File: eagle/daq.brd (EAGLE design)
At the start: 76.2 x 65.4 mm, 109 parts

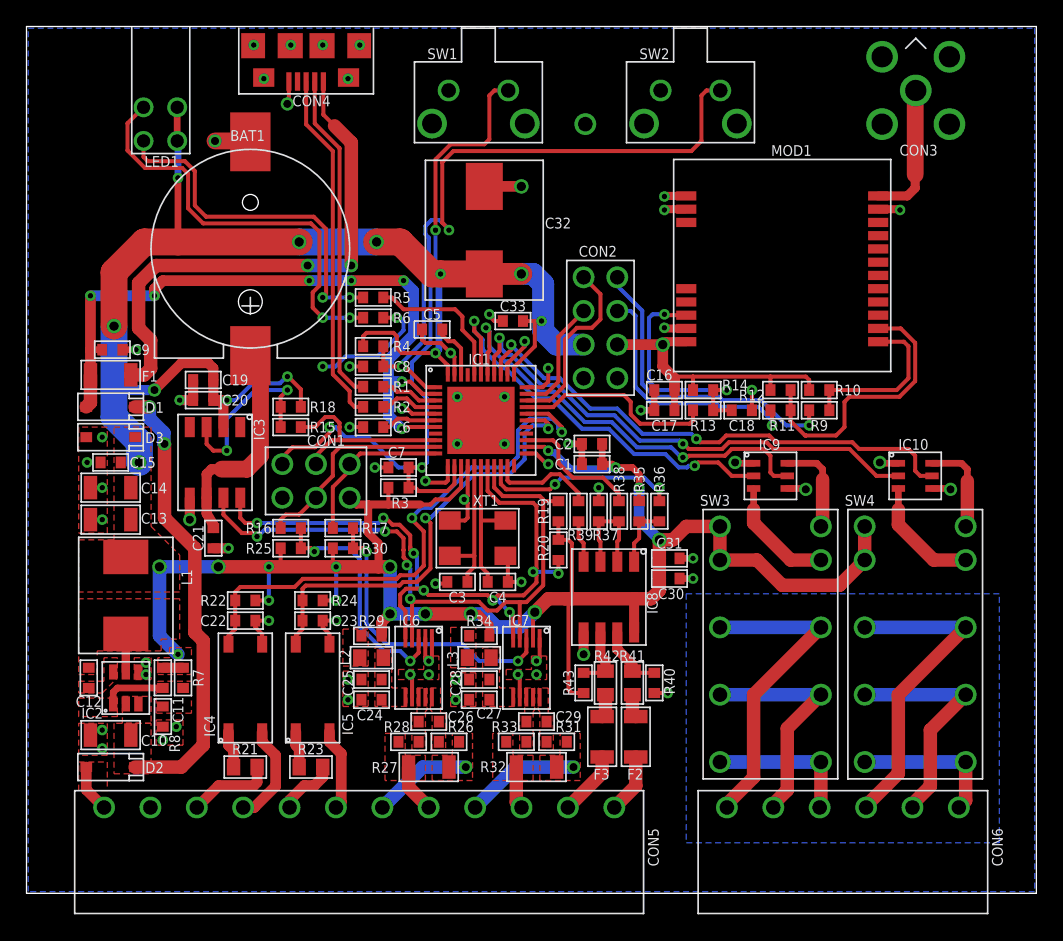
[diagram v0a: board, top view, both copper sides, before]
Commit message: do
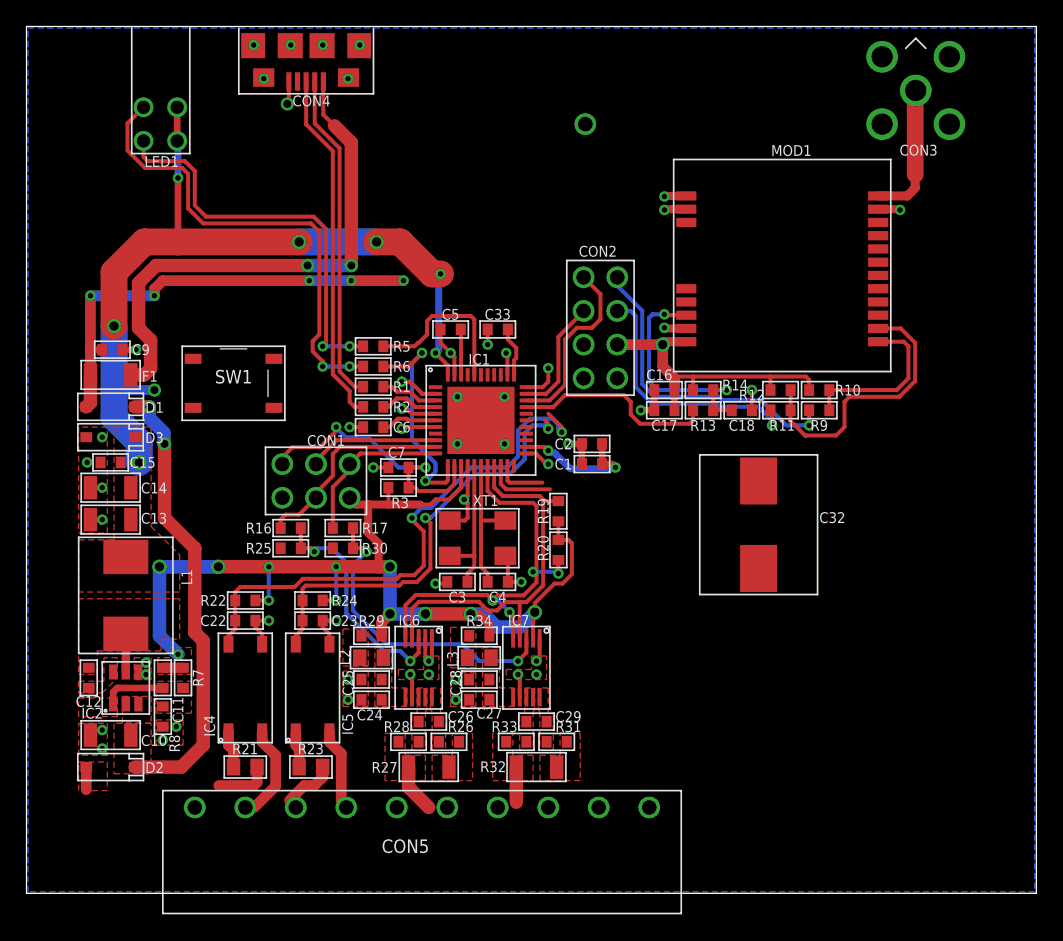
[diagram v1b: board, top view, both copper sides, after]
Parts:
- removed BAT1: (no value), myparts:BAT-1220-BC501SM
- removed C19, C20, C21, C30, C31, C8, R15, R18, R35, R36, R37, R38, R39, R4, R40, R43: (no value), myparts:0603
- removed CON6: (no value), myparts:KF2EDGR-3.5-6P
- removed F2, F3: (no value), myparts:1206
- removed IC10, IC9: (no value), myparts:SC74-6
- removed IC3, IC8: (no value), myparts:SOIC-8
- removed R41, R42: (no value), myparts:0805
- removed SW2: (no value), myparts:B3F-3150-52-55
- removed SW3, SW4: (no value), myparts:HFD2-L2
- CON5: device myparts:KF2EDGR-3.5-12P -> myparts:15EDGRC-3.81-10P
- SW1: device myparts:B3F-3150-52-55 -> myparts:BUTTON-4P-SMD-5X5
- moved C32 30.4 mm to (55.2, 27.8)
- moved SW1 28.8 mm to (15.6, 38.5), turned to 0 degrees
- moved CON5 4.74 mm to (29.8, 6.48)
- moved R5 3.68 mm to (26.2, 41.3)
- moved R6 3.68 mm to (26.2, 39.8)
- moved C5 1.40 mm to (32.0, 42.5)
- moved C33 1.31 mm to (35.6, 42.5)
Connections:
- removed net N$24: IC1.36, IC10.5
- removed net N$26: IC9.6, SW3.L1-
- removed net N$28: IC9.3, SW3.L2-
- removed net N$29: C8.1, IC1.1, R4.1, SW2.1
- removed net N$38: IC1.37, IC10.2
- removed net N$39: CON6.1, SW4.NO1, SW4.NO2
- removed net N$46: CON5.2, F3.1
- removed net N$47: IC8.1, R35.2, R36.2
- removed net N$48: IC8.4, R39.2
- removed net N$51: IC8.7, R40.2, R41.2
- removed net N$52: IC8.6, R42.2, R43.2
- removed net N$53: IC8.2, IC8.3, R37.2, R38.2
- removed net N$54: F3.2, R42.1
- removed net N$58: BAT1.+, C21.2, IC3.6
- removed net N$60: CON5.1, F2.1
- removed net N$61: IC1.20, R36.1
- removed net N$62: IC1.21, R39.1
- removed net N$63: IC1.25, R38.1
- removed net N$64: IC10.6, SW4.L1-
- removed net N$67: CON6.2, SW4.NC1, SW4.NC2
- removed net N$70: IC3.3, R15.1, R18.2
- removed net N$74: CON6.3, SW4.C1, SW4.C2
- removed net N$80: F2.2, R41.1
- removed net N$82: IC10.3, SW4.L2-
- removed net N$86: CON6.4, SW3.NO1, SW3.NO2
- removed net N$87: CON6.5, SW3.NC1, SW3.NC2
- removed net N$88: CON6.6, SW3.C1, SW3.C2
- removed net N$90: IC1.38, IC9.5
- removed net N$91: IC1.39, IC9.2
- net GND: now also CON5.2; no longer BAT1.-, C19.1, C20.1, C21.1, C30.1, C31.1, C8.2, CON5.11, IC10.1, IC10.4, IC3.5, IC8.5, IC9.1, IC9.4, R37.1, R40.1, SW1.4, SW2.2, SW2.3, SW2.4
- net N$30: now also CON5.9; no longer CON5.4
- net N$32: now also IC1.21; no longer IC1.28
- net N$35: now also IC1.20; no longer IC1.29
- net N$40: now also CON5.10; no longer CON5.3
- net N$41: now also SW1.4
- net N$45: no longer R15.2
- net N$49: now also CON5.6; no longer CON5.7
- net N$50: now also CON5.4; no longer CON5.9
- net N$55: now also CON5.5; no longer CON5.8
- net N$59: now also CON5.7; no longer CON5.6
- net N$73: no longer IC3.8
- net N$79: no longer IC3.7
- net N$81: now also CON5.8; no longer CON5.5
- net N$85: now also CON5.3; no longer CON5.10
- net VCC: no longer C19.2, C20.2, C30.2, C31.2, IC3.2, IC8.8, R18.1, R35.1, R4.2, R43.1, SW3.L1+, SW3.L2+, SW4.L1+, SW4.L2+
- net VEXT: now also CON5.1; no longer CON5.12
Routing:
- net VCC: track 260.1 -> 159.7 mm, vias 28 -> 22
- net N$29: track 50.5 -> 0.00 mm, vias 2 -> 0
- net N$24: track 39.6 -> 0.00 mm, vias 2 -> 0
- net N$38: track 38.2 -> 0.00 mm, vias 2 -> 0
- net N$41: track 55.4 -> 21.7 mm, vias 3 -> 2
- net N$90: track 33.0 -> 0.00 mm, vias 2 -> 0
- net N$91: track 31.4 -> 0.00 mm, vias 2 -> 0
- net GND: track 98.0 -> 72.1 mm, vias 68 -> 53
- net N$74: track 24.3 -> 0.00 mm
- net N$88: track 24.1 -> 0.00 mm
- net N$79: track 51.1 -> 29.5 mm, vias 4 -> 0
- net N$73: track 53.5 -> 32.2 mm, vias 8 -> 4
- net N$67: track 17.8 -> 0.00 mm
- net N$87: track 17.6 -> 0.00 mm
- net N$58: track 16.7 -> 0.00 mm
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- removed copper zone on layer 16, net GNDX

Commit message: do
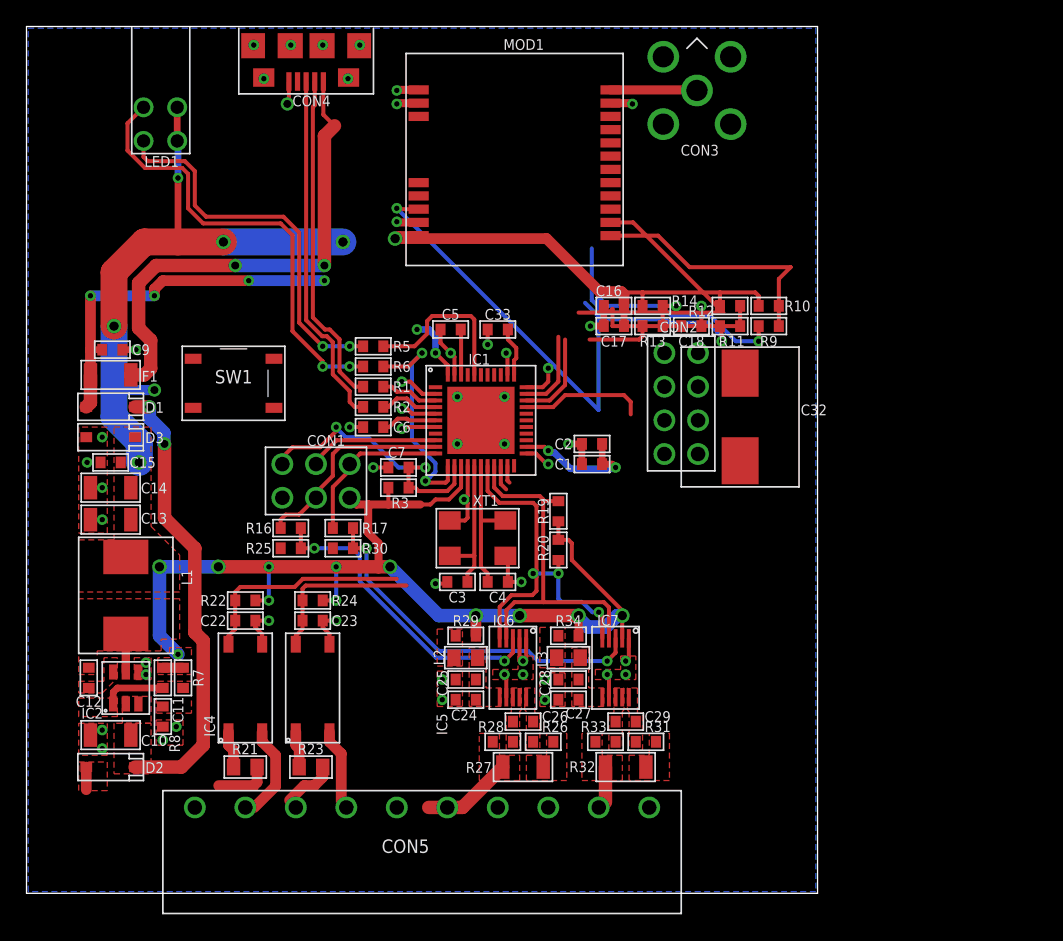
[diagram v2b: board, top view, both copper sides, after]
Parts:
- moved MOD1 21.7 mm to (36.8, 55.4)
- moved CON3 16.5 mm to (50.6, 60.6)
- moved CON2 8.36 mm to (48.1, 40.8)
- moved C32 8.25 mm to (53.8, 35.9)
- moved C16 7.41 mm to (44.3, 44.3)
- moved C17 7.41 mm to (44.3, 42.8)
- moved C18 7.41 mm to (50.2, 42.8)
- moved R10 7.41 mm to (56.0, 44.3)
- moved R11 7.41 mm to (53.1, 42.8)
- moved R12 7.41 mm to (53.1, 44.3)
- moved R13 7.41 mm to (47.2, 42.8)
- moved R14 7.41 mm to (47.2, 44.3)
- moved R9 7.41 mm to (56.0, 42.8)
- moved C26 7.11 mm to (37.5, 13.0)
- moved IC6 7.11 mm to (36.7, 17.0)
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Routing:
- net N$35: track 46.4 -> 18.7 mm, vias 2 -> 0
- net N$2: track 17.8 -> 41.8 mm
- net N$32: track 36.6 -> 15.4 mm, vias 2 -> 0
- net N$7: track 21.1 -> 35.1 mm
- net N$13: track 23.9 -> 36.6 mm
- net VCC: track 159.7 -> 151.2 mm
- net N$11: track 13.8 -> 6.83 mm
- net N$16: track 19.8 -> 12.9 mm
- net N$6: track 12.7 -> 19.4 mm
- net UVCC: track 39.3 -> 33.3 mm, vias 7 -> 6
- net N$23: track 17.7 -> 23.5 mm
- net N$14: track 23.9 -> 18.9 mm
- net N$25: track 23.5 -> 27.5 mm
- net N$4: track 10.4 -> 6.54 mm
- net N$73: track 32.2 -> 28.7 mm, vias 4 -> 3
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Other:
- board size 76.2 x 65.4 mm -> 59.7 x 65.4 mm

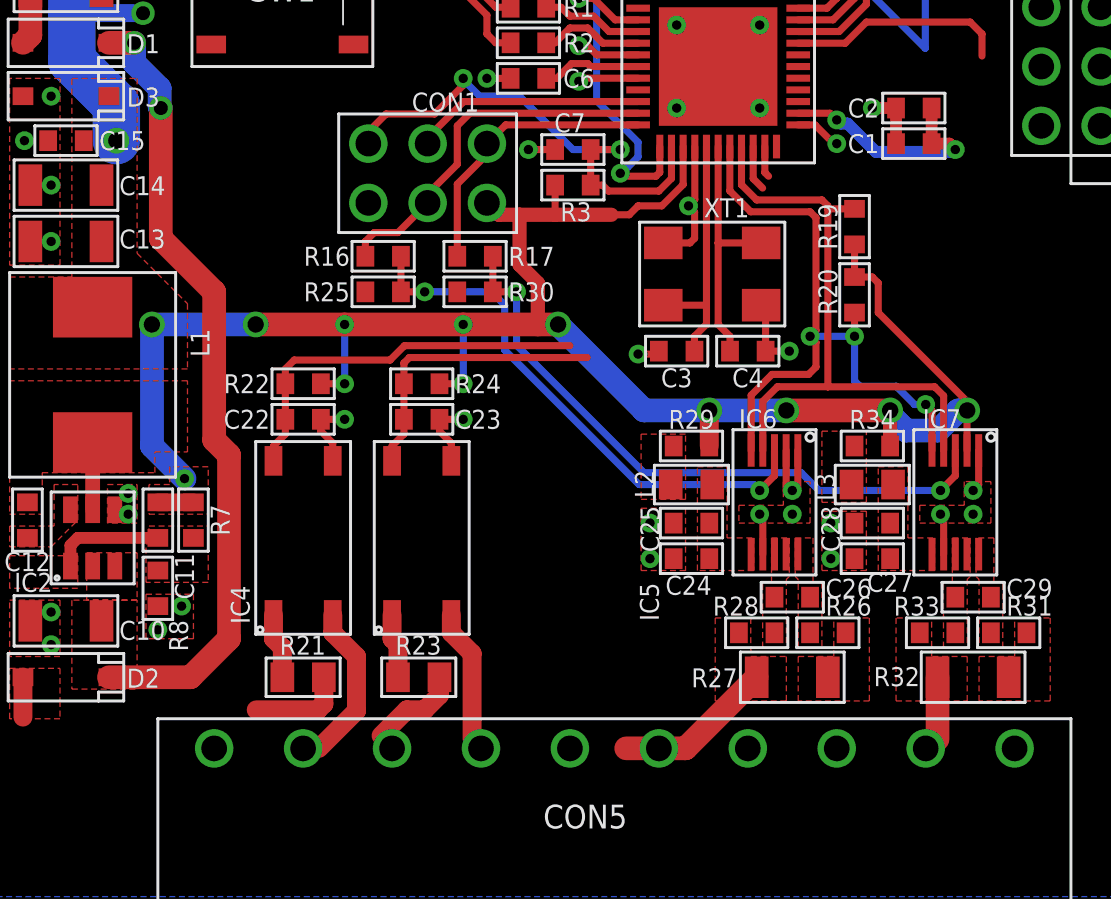
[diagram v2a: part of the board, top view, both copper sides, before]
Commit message: do
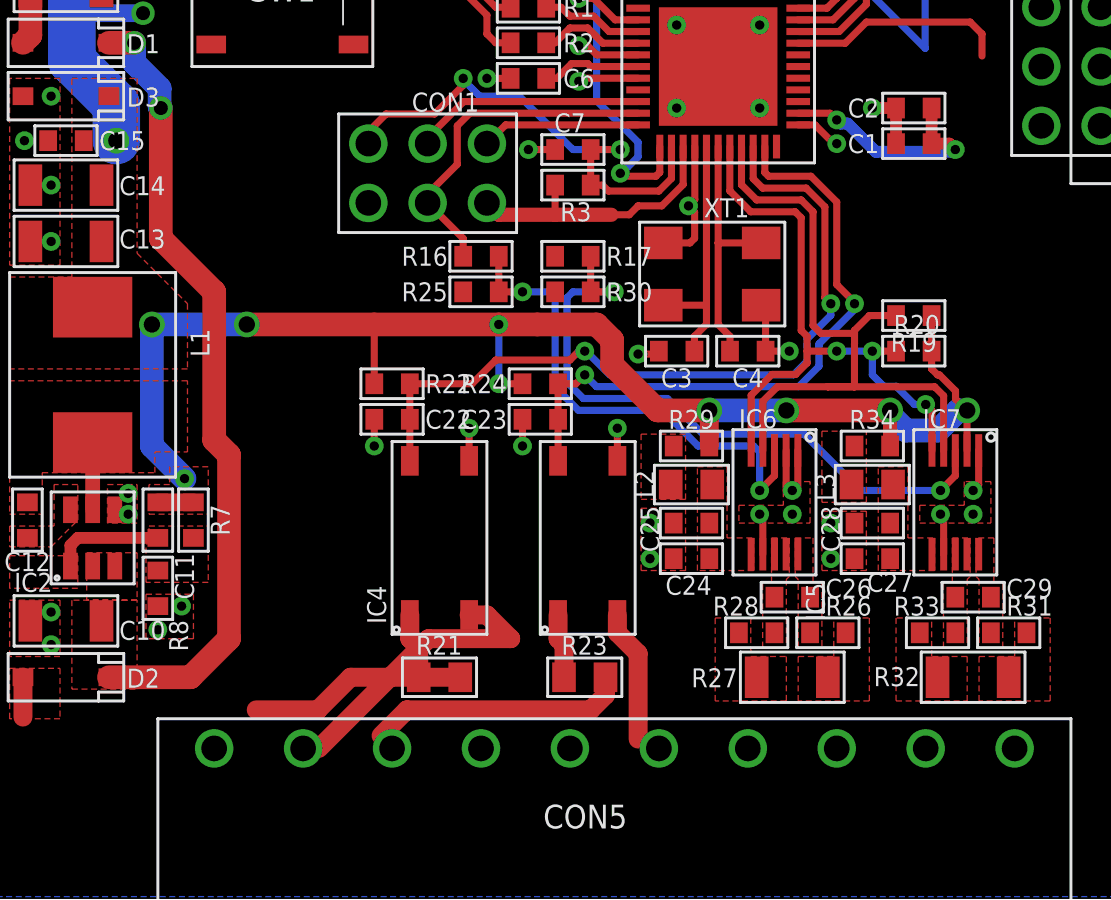
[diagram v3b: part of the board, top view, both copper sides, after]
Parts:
- moved IC5 7.11 mm to (28.7, 15.5)
- moved R23 7.11 mm to (28.6, 9.53)
- moved IC4 5.84 mm to (22.4, 15.5)
- moved R21 5.84 mm to (22.4, 9.53)
- moved C23 5.08 mm to (26.7, 20.6), turned to 0 degrees
- moved R24 5.08 mm to (26.7, 22.1), turned to 0 degrees
- moved R19 4.58 mm to (42.7, 25.0), turned to 180 degrees
- moved R16 4.19 mm to (24.1, 27.6)
- moved R17 4.19 mm to (28.1, 27.6)
- moved R25 4.19 mm to (24.1, 26.0)
- moved R30 4.19 mm to (28.1, 26.0)
- moved C22 3.81 mm to (20.3, 20.6), turned to 0 degrees
- moved R22 3.81 mm to (20.3, 22.1), turned to 0 degrees
- moved R20 3.50 mm to (42.7, 23.5), turned to 180 degrees
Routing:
- net N$35: track 18.7 -> 33.6 mm, vias 0 -> 2
- net N$32: track 15.4 -> 27.9 mm, vias 0 -> 2
- net VCC: track 151.2 -> 140.0 mm, vias 22 -> 19
- net N$55: track 3.98 -> 11.1 mm
- net N$81: track 6.85 -> 0.00 mm
- net N$50: track 6.81 -> 12.4 mm
- net N$3: track 12.2 -> 6.81 mm
- net N$85: track 4.15 -> 9.32 mm
- net N$79: track 27.2 -> 30.2 mm
- net N$40: track 2.66 -> 0.00 mm
- net N$23: track 23.5 -> 21.4 mm
- net N$73: track 28.7 -> 26.8 mm
- net N$9: track 15.8 -> 14.7 mm
- net GND: track 72.1 -> 71.2 mm, vias 52 -> 54
- net N$25: track 27.5 -> 28.2 mm

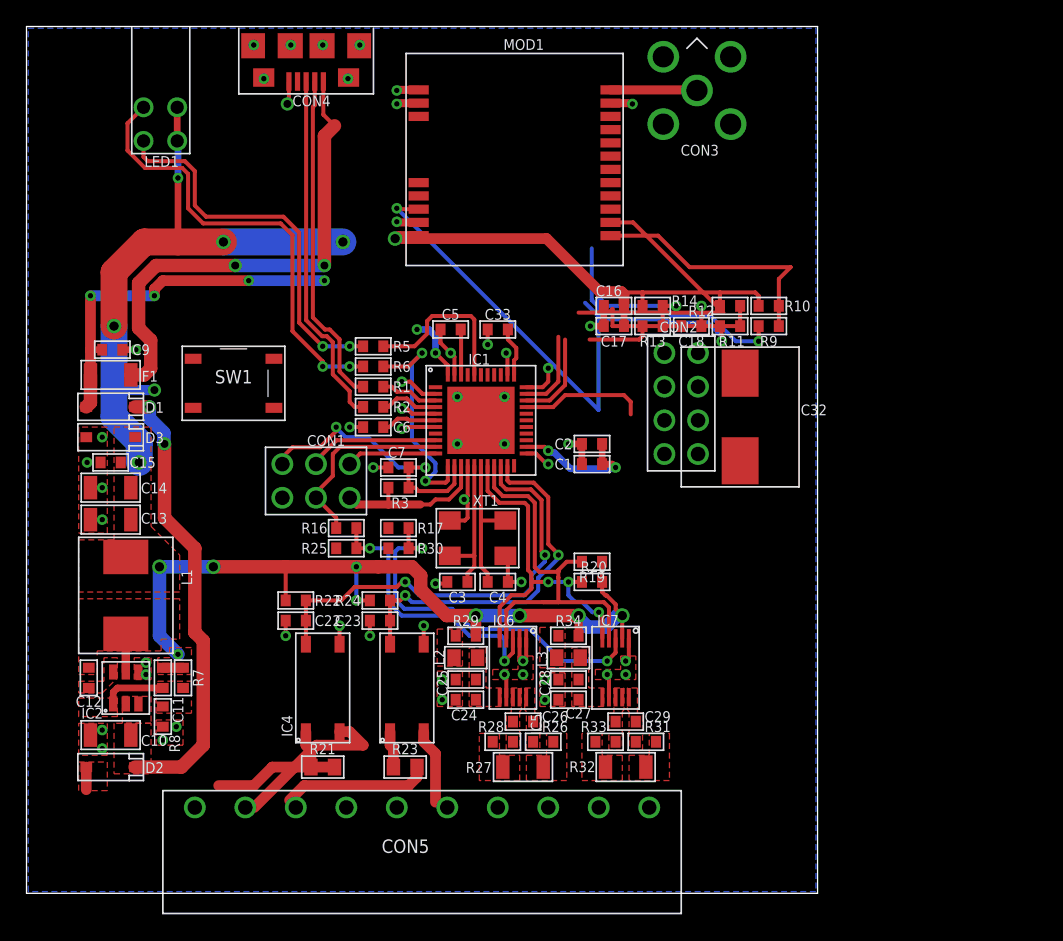
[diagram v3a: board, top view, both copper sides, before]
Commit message: do
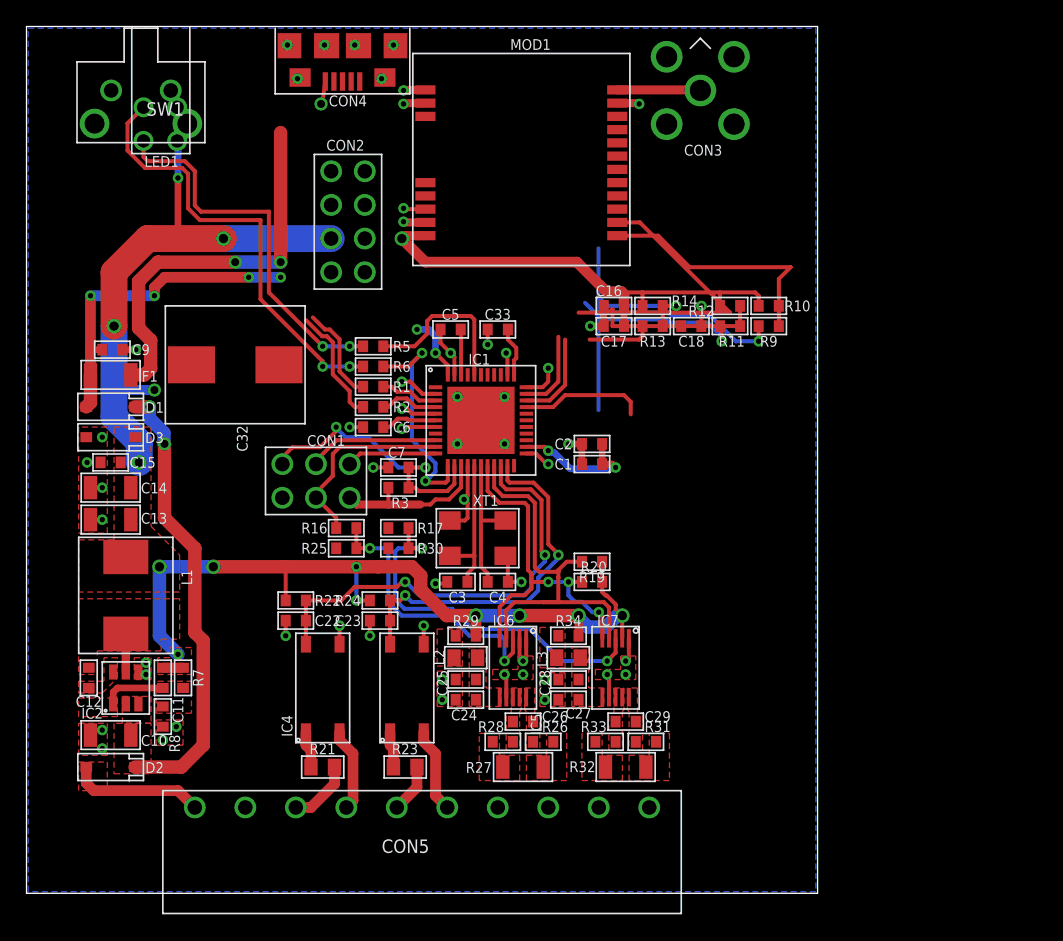
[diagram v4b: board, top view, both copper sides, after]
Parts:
- SW1: device myparts:BUTTON-4P-SMD-5X5 -> myparts:B3F-3150-52-55
- moved C32 38.3 mm to (15.7, 39.9), turned to 270 degrees
- moved CON2 28.6 mm to (23.0, 54.5)
- moved SW1 23.2 mm to (8.64, 60.6), turned to 180 degrees
- moved CON4 2.74 mm to (23.8, 65.4)
- moved MOD1 0.51 mm to (37.3, 55.4)
- moved CON3 0.25 mm to (50.8, 60.6)
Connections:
- net GND: now also SW1.4
- net N$41: no longer SW1.4
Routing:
- net N$2: track 41.8 -> 20.3 mm
- net N$19: track 26.9 -> 8.90 mm
- net N$18: track 25.2 -> 7.38 mm
- net VEXT: track 1.71 -> 10.2 mm
- net N$56: track 37.6 -> 29.8 mm
- net N$55: track 11.1 -> 3.68 mm
- net N$50: track 12.4 -> 6.35 mm
- net N$85: track 9.32 -> 4.93 mm
- net UVCC: track 33.3 -> 30.2 mm
- net GND: track 71.2 -> 72.4 mm
- net VCC: track 140.0 -> 139.0 mm, vias 19 -> 18
- net N$49: track 5.69 -> 6.45 mm
- net N$8: track 34.3 -> 33.5 mm
- net N$13: track 36.6 -> 36.1 mm
- net N$7: track 35.1 -> 35.6 mm
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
